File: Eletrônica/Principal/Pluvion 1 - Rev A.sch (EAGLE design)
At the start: 46 parts, among them IC1 REG1117, J3 22-05-7048-04, J4 22-05-7048-04, J5 22-05-7028-02, Q1 PFET, Q2 NFET, Q3 S8050, Q4 S8050, SW1 Reset

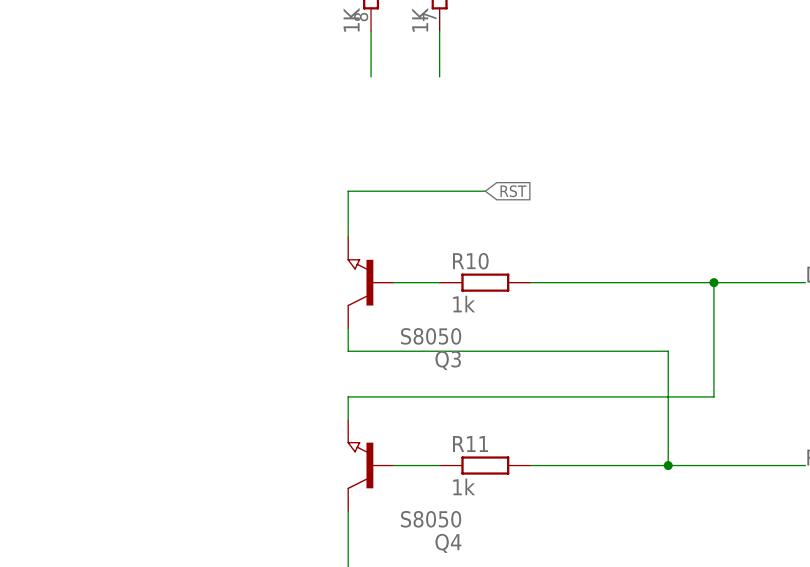
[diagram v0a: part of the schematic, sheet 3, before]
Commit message: Pluvion 1 Rev C
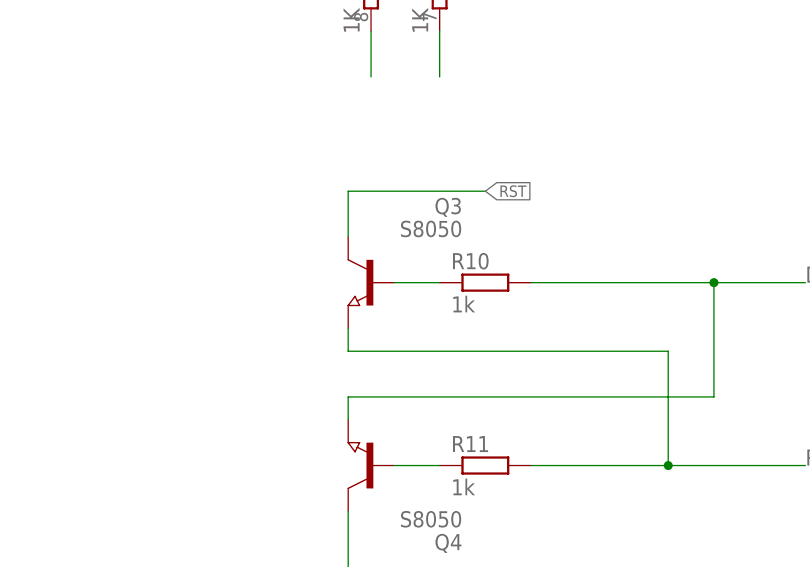
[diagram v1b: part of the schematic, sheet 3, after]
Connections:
- net RST: now also Q3.C; no longer Q3.E
- net RTS: now also Q3.E; no longer Q3.C
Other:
- moved on the sheet: Q3
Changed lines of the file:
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@@
 <grid distance="0.1" unitdist="inch" unit="inch" style="lines" multiple="1" display="no" altdistance="0.01" altunitdist="inch" altunit="inch"/>
 <layers>
-<layer number="1" name="Top" color="4" fill="1" visible="yes" active="no"/>
-<layer number="2" name="Route2" color="1" fill="3" visible="yes" active="no"/>
-<layer number="3" name="Route3" color="4" fill="3" visible="yes" active="no"/>
-<layer number="4" name="Route4" color="1" fill="4" visible="yes" active="no"/>
-<layer number="5" name="Route5" color="4" fill="4" visible="yes" active="no"/>
-<layer number="6" name="Route6" color="1" fill="8" visible="yes" active="no"/>
-<layer number="7" name="Route7" color="4" fill="8" visible="yes" active="no"/>
-<layer number="8" name="Route8" color="1" fill="2" visible="yes" active="no"/>
-<layer number="9" name="Route9" color="4" fill="2" visible="yes" active="no"/>
-<layer number="10" name="Route10" color="1" fill="7" visible="yes" active="no"/>
-<layer number="11" name="Route11" color="4" fill="7" visible="yes" active="no"/>
-<layer number="12" name="Route12" color="1" fill="5" visible="yes" active="no"/>
-<layer number="13" name="Route13" color="4" fill="5" visible="yes" active="no"/>
-<layer number="14" name="Route14" color="1" fill="6" visible="yes" active="no"/>
-<layer number="15" name="Route15" color="4" fill="6" visible="yes" active="no"/>
-<layer number="16" name="Bottom" color="1" fill="1" visible="yes" active="no"/>
-<layer number="17" name="Pads" color="2" fill="1" visible="yes" active="no"/>
-<layer number="18" name="Vias" color="2" fill="1" visible="yes" active="no"/>
-<layer number="19" name="Unrouted" color="6" fill="1" visible="yes" active="no"/>
-<layer number="20" name="Dimension" color="15" fill="1" visible="yes" active="no"/>
-<layer number="21" name="tPlace" color="7" fill="1" visible="yes" active="no"/>
-<layer number="22" name="bPlace" color="7" fill="1" visible="yes" active="no"/>
-<layer number="23" name="tOrigins" color="15" fill="1" visible="yes" active="no"/>
-<layer number="24" name="bOrigins" color="15" fill="1" visible="yes" active="no"/>
-<layer number="25" name="tNames" color="7" fill="1" visible="yes" active="no"/>
-<layer number="26" name="bNames" color="7" fill="1" visible="yes" active="no"/>
-<layer number="27" name="tValues" color="7" fill="1" visible="yes" active="no"/>
-<layer number="28" name="bValues" color="7" fill="1" visible="yes" active="no"/>
+<layer number="1" name="Top" color="4" fill="1" visible="no" active="no"/>
+<layer number="2" name="Route2" color="1" fill="3" visible="no" active="no"/>
+<layer number="3" name="Route3" color="4" fill="3" visible="no" active="no"/>
+<layer number="4" name="Route4" color="1" fill="4" visible="no" active="no"/>
+<layer number="5" name="Route5" color="4" fill="4" visible="no" active="no"/>
+<layer number="6" name="Route6" color="1" fill="8" visible="no" active="no"/>
+<layer number="7" name="Route7" color="4" fill="8" visible="no" active="no"/>
+<layer number="8" name="Route8" color="1" fill="2" visible="no" active="no"/>
+<layer number="9" name="Route9" color="4" fill="2" visible="no" active="no"/>
+<layer number="10" name="Route10" color="1" fill="7" visible="no" active="no"/>
+<layer number="11" name="Route11" color="4" fill="7" visible="no" active="no"/>
+<layer number="12" name="Route12" color="1" fill="5" visible="no" active="no"/>
+<layer number="13" name="Route13" color="4" fill="5" visible="no" active="no"/>
+<layer number="14" name="Route14" color="1" fill="6" visible="no" active="no"/>
+<layer number="15" name="Route15" color="4" fill="6" visible="no" active="no"/>
+<layer number="16" name="Bottom" color="1" fill="1" visible="no" active="no"/>
+<layer number="17" name="Pads" color="2" fill="1" visible="no" active="no"/>
+<layer number="18" name="Vias" color="2" fill="1" visible="no" active="no"/>
+<layer number="19" name="Unrouted" color="6" fill="1" visible="no" active="no"/>
+<layer number="20" name="Dimension" color="15" fill="1" visible="no" active="no"/>
+<layer number="21" name="tPlace" color="7" fill="1" visible="no" active="no"/>
+<layer number="22" name="bPlace" color="7" fill="1" visible="no" active="no"/>
+<layer number="23" name="tOrigins" color="15" fill="1" visible="no" active="no"/>
+<layer number="24" name="bOrigins" color="15" fill="1" visible="no" active="no"/>
+<layer number="25" name="tNames" color="7" fill="1" visible="no" active="no"/>
+<layer number="26" name="bNames" color="7" fill="1" visible="no" active="no"/>
+<layer number="27" name="tValues" color="7" fill="1" visible="no" active="no"/>
+<layer number="28" name="bValues" color="7" fill="1" visible="no" active="no"/>
 <layer number="29" name="tStop" color="7" fill="3" visible="no" active="no"/>
 <layer number="30" name="bStop" color="7" fill="6" visible="no" active="no"/>
@@
 <layer number="35" name="tGlue" color="7" fill="4" visible="no" active="no"/>
 <layer number="36" name="bGlue" color="7" fill="5" visible="no" active="no"/>
-<layer number="37" name="tTest" color="7" fill="1" visible="yes" active="no"/>
-<layer number="38" name="bTest" color="7" fill="1" visible="yes" active="no"/>
+<layer number="37" name="tTest" color="7" fill="1" visible="no" active="no"/>
+<layer number="38" name="bTest" color="7" fill="1" visible="no" active="no"/>
 <layer number="39" name="tKeepout" color="4" fill="11" visible="no" active="no"/>
 <layer number="40" name="bKeepout" color="1" fill="11" visible="no" active="no"/>
@@
 <layer number="44" name="Drills" color="7" fill="1" visible="no" active="no"/>
 <layer number="45" name="Holes" color="7" fill="1" visible="no" active="no"/>
-<layer number="46" name="Milling" color="3" fill="1" visible="yes" active="no"/>
-<layer number="47" name="Measures" color="7" fill="1" visible="yes" active="no"/>
-<layer number="48" name="Document" color="7" fill="1" visible="yes" active="no"/>
-<layer number="49" name="Reference" color="7" fill="1" visible="yes" active="no"/>
-<layer number="50" name="dxf" color="7" fill="1" visible="yes" active="no"/>
-<layer number="51" name="tDocu" color="7" fill="1" visible="yes" active="no"/>
-<layer number="52" name="bDocu" color="7" fill="1" visible="yes" active="no"/>
-<layer number="53" name="tGND_GNDA" color="7" fill="9" visible="yes" active="no"/>
-<layer number="54" name="bGND_GNDA" color="1" fill="9" visible="yes" active="no"/>
-<layer number="56" name="wert" color="7" fill="1" visible="yes" active="no"/>
-<layer number="57" name="tCAD" color="7" fill="1" visible="yes" active="no"/>
+<layer number="46" name="Milling" color="3" fill="1" visible="no" active="no"/>
+<layer number="47" name="Measures" color="7" fill="1" visible="no" active="no"/>
+<layer number="48" name="Document" color="7" fill="1" visible="no" active="no"/>
+<layer number="49" name="Reference" color="7" fill="1" visible="no" active="no"/>
+<layer number="50" name="dxf" color="7" fill="1" visible="no" active="no"/>
+<layer number="51" name="tDocu" color="7" fill="1" visible="no" active="no"/>
+<layer number="52" name="bDocu" color="7" fill="1" visible="no" active="no"/>
+<layer number="53" name="tGND_GNDA" color="7" fill="9" visible="no" active="no"/>
+<layer number="54" name="bGND_GNDA" color="1" fill="9" visible="no" active="no"/>
+<layer number="56" name="wert" color="7" fill="1" visible="no" active="no"/>
+<layer number="57" name="tCAD" color="7" fill="1" visible="no" active="no"/>
 <layer number="90" name="Modules" color="5" fill="1" visible="yes" active="yes"/>
 <layer number="91" name="Nets" color="2" fill="1" visible="yes" active="yes"/>
@@
 <instance part="SW1" gate="1" x="20.32" y="43.18" rot="MR0"/>
 <instance part="GND7" gate="1" x="10.16" y="35.56"/>
-<instance part="Q3" gate="G$1" x="22.86" y="-60.96" rot="R180"/>
+<instance part="Q3" gate="G$1" x="22.86" y="-60.96" rot="MR0"/>
 <instance part="Q4" gate="G$1" x="22.86" y="-81.28" rot="R180"/>
 <instance part="+3V4" gate="G$1" x="-43.18" y="33.02"/>
@@
 <net name="RST" class="0">
 <segment>
-<pinref part="Q3" gate="G$1" pin="E"/>
-<wire x1="20.32" y1="-55.88" x2="20.32" y2="-50.8" width="0.1524" layer="91"/>
 <wire x1="20.32" y1="-50.8" x2="35.56" y2="-50.8" width="0.1524" layer="91"/>
 <label x="35.56" y="-50.8" size="1.27" layer="95" xref="yes"/>
+<pinref part="Q3" gate="G$1" pin="C"/>
+<wire x1="20.32" y1="-55.88" x2="20.32" y2="-50.8" width="0.1524" layer="91"/>
 </segment>
 <segment>
@@
 <segment>
 <wire x1="40.64" y1="-81.28" x2="55.88" y2="-81.28" width="0.1524" layer="91"/>
-<pinref part="Q3" gate="G$1" pin="C"/>
 <wire x1="55.88" y1="-81.28" x2="71.12" y2="-81.28" width="0.1524" layer="91"/>
-<wire x1="20.32" y1="-66.04" x2="20.32" y2="-68.58" width="0.1524" layer="91"/>
 <wire x1="20.32" y1="-68.58" x2="55.88" y2="-68.58" width="0.1524" layer="91"/>
 <wire x1="55.88" y1="-68.58" x2="55.88" y2="-81.28" width="0.1524" layer="91"/>
@@
 <label x="71.12" y="-81.28" size="1.778" layer="95"/>
 <pinref part="R11" gate="G$1" pin="2"/>
-</segment>
-<segment>
+<pinref part="Q3" gate="G$1" pin="E"/>
+<wire x1="20.32" y1="-66.04" x2="20.32" y2="-68.58" width="0.1524" layer="91"/>
+</segment>
+<segment>
